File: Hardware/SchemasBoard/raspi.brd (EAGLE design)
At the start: 14.9 x 30.5 mm, 7 parts

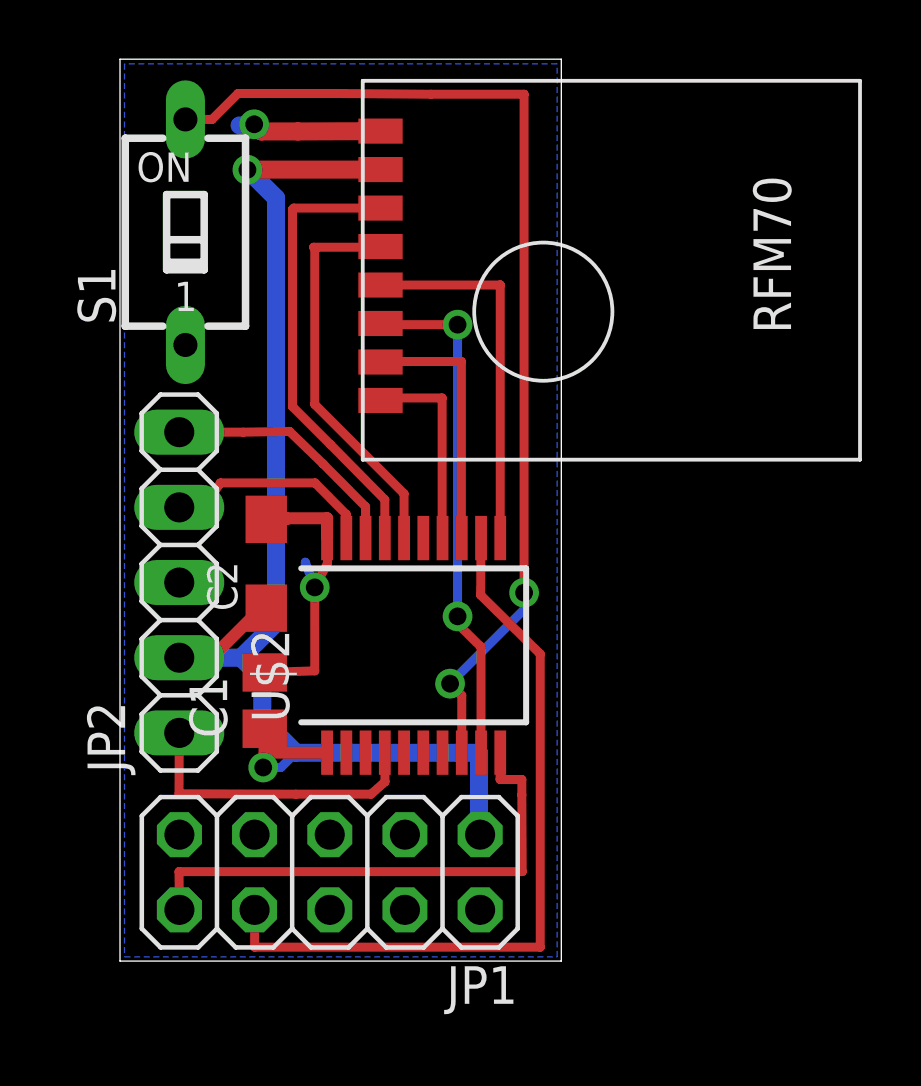
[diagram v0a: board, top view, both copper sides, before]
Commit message: aa
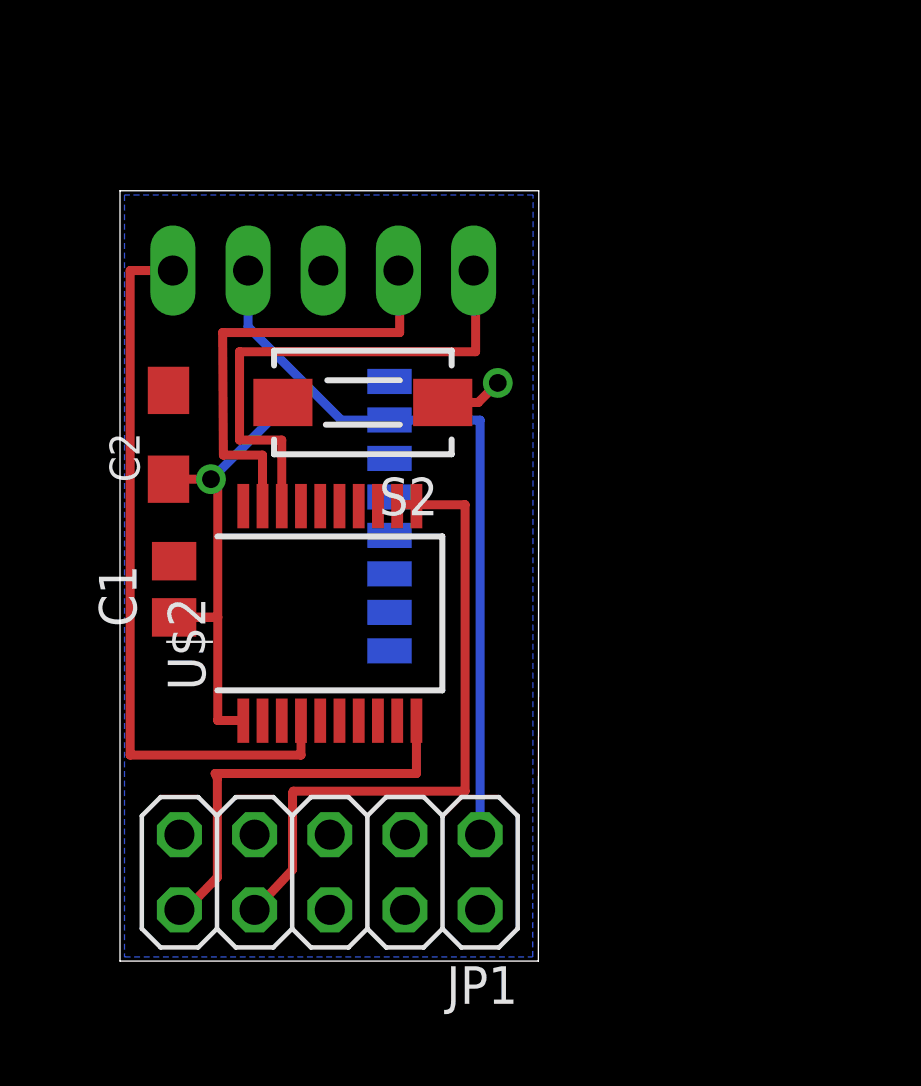
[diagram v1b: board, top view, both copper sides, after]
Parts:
- removed S1: (no value), switch-dil:SD4-01
- added S2: DTSM-3, switch-tact:DTSM-3
- moved U$1 29.5 mm to (-5.19, 19.5), flipped to the bottom
- moved JP2 11.6 mm to (6.87, 23.3), flipped to the bottom, turned to 180 degrees
- moved C2 5.47 mm to (1.64, 17.8)
- moved C1 4.85 mm to (1.83, 12.6)
- moved U$2 3.03 mm to (7.09, 11.7)
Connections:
- net GND: now also S2.1; no longer S1.1
- net N$28: now also S2.2, U$2.3; no longer S1.2, U$2.8
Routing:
- net N$28: track 35.3 -> 0.00 mm, vias 2 -> 0
- net N$23: track 17.4 -> 0.00 mm, vias 2 -> 0
- net N$16: track 15.4 -> 0.00 mm
- net N$25: track 10.2 -> 24.7 mm
- net N$20: track 13.4 -> 0.00 mm
- net N$22: track 12.6 -> 0.00 mm
- net GND: track 15.0 -> 2.49 mm, vias 2 -> 1
- net N$19: track 8.40 -> 17.4 mm
- net N$12: track 8.73 -> 0.00 mm
- net N$18: track 7.33 -> 15.3 mm
- net N$21: track 6.91 -> 0.00 mm
- net N$33: track 17.6 -> 13.9 mm
- net N$34: track 25.6 -> 22.4 mm
- net VDD: track 46.3 -> 43.2 mm, vias 2 -> 1
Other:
- board size 14.9 x 30.5 mm -> 14.1 x 26 mm
